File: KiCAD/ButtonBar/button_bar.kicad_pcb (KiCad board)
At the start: 2 copper layers, 14 parts, among them P1 Buttons, SW1 SW_UP, SW2 SW_DN, SW3 SW_OK, SW4 SW_LT, SW5 SW_RT, SW6 RESET

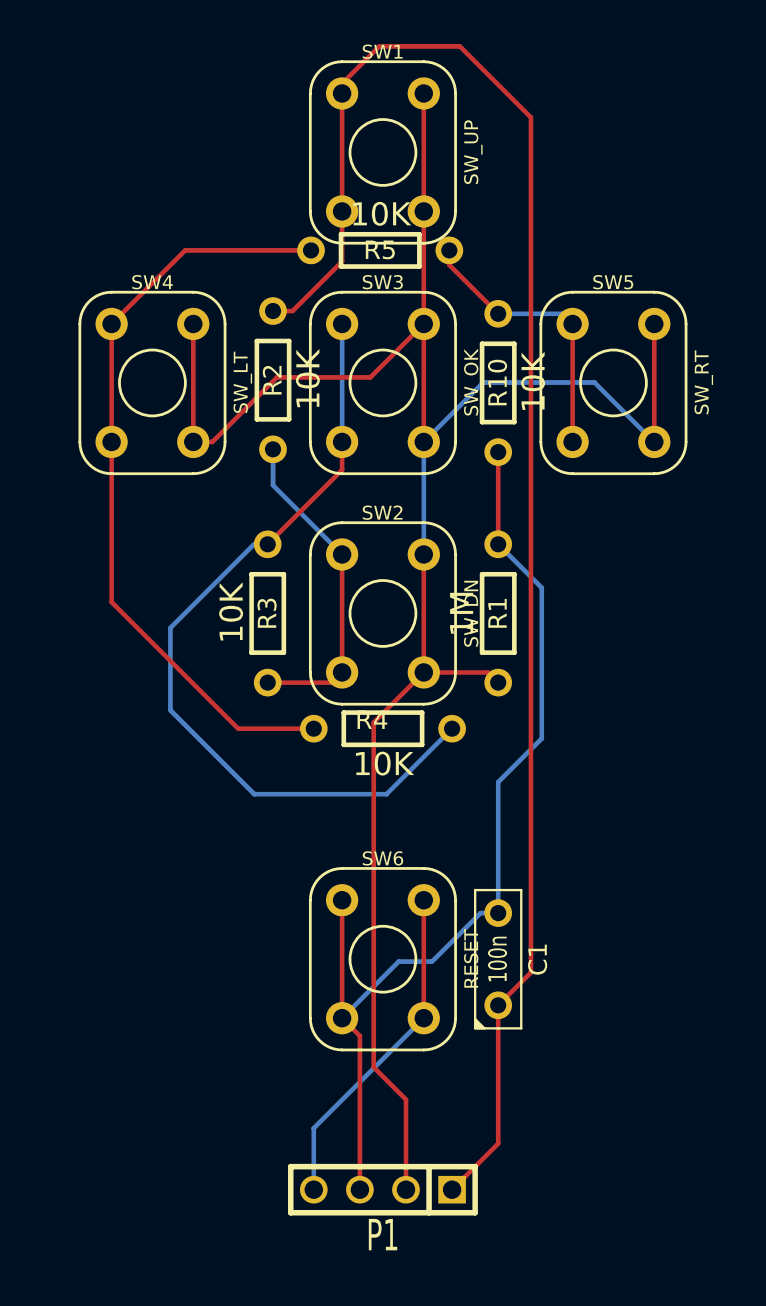
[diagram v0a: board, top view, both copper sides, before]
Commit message: button board pcb update ajm
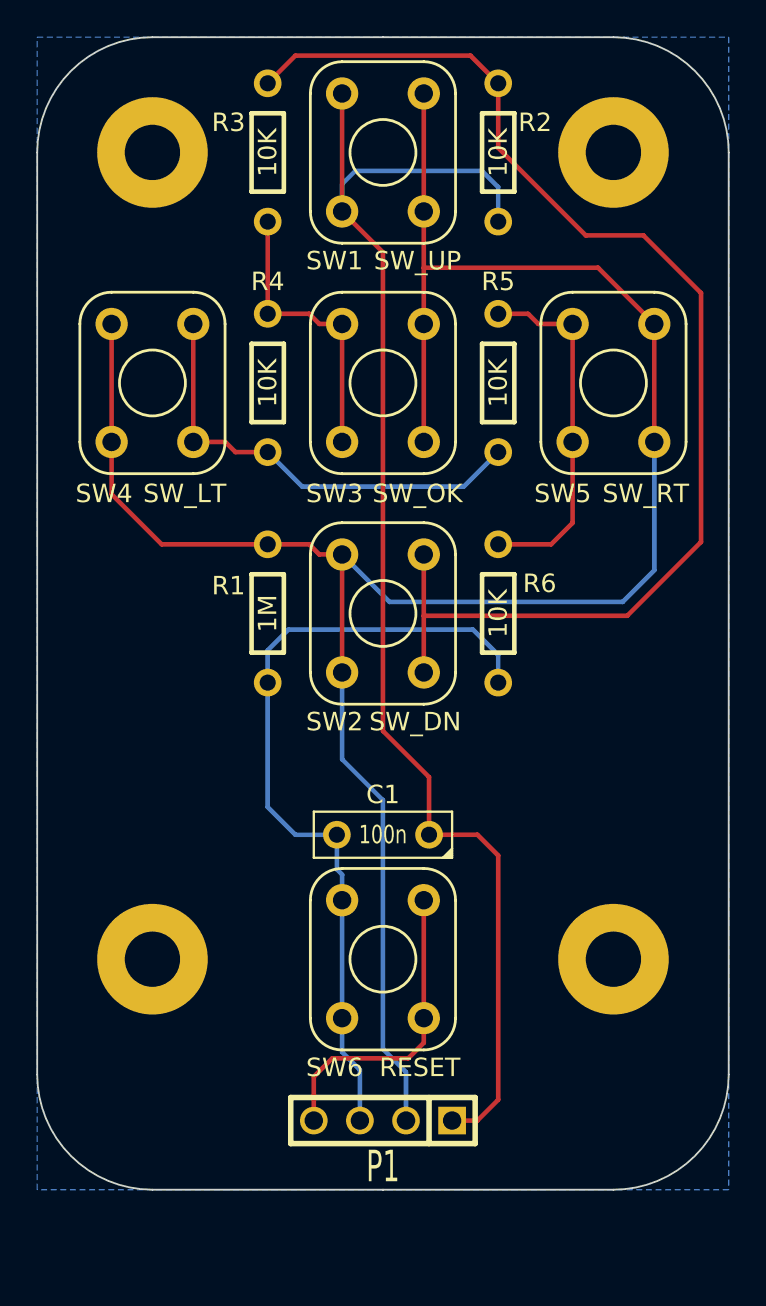
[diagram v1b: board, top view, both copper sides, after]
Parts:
- added H1: CONN_1, vite_3mm, F.Cu at (190.5, 63.5)
- added H2: CONN_1, vite_3mm, F.Cu at (215.9, 63.5)
- added H3: CONN_1, vite_3mm, F.Cu at (215.9, 108.0)
- added H4: CONN_1, vite_3mm, F.Cu at (190.5, 108.0)
- moved R3 25.4 mm to (196.8, 63.5), turned to 90 degrees
- moved R4 20.1 mm to (196.8, 76.2), turned to 90 degrees
- moved R2 17.6 mm to (209.6, 63.5), turned to 270 degrees
- moved R1 12.7 mm to (196.8, 88.9), turned to 90 degrees
- moved R6 12.7 mm to (209.6, 88.9)
- moved R5 9.78 mm to (209.6, 76.2), turned to 270 degrees
- moved C1 9.35 mm to (203.2, 101.1), turned to 180 degrees
- moved P1 3.81 mm to (203.2, 116.8)
- turned SW2 to 180 degrees
- turned SW4 to 180 degrees
- renumbered R10 to R6
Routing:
- net N-000004: track 18.2 -> 69.2 mm
- net N-000001: track 44.6 -> 15.9 mm
- net N-000003: track 42.0 -> 25.1 mm
- net /PWR: track 88.5 -> 76.3 mm
- net /SW: track 110.4 -> 121.9 mm
- net GND: track 54.7 -> 44.6 mm
- net N-000002: track 15.4 -> 19.9 mm
- net /RST: track 18.5 -> 17.1 mm
- added copper zone on B.Cu, net GND
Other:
- board outline added: 38.1 x 63.5 mm
